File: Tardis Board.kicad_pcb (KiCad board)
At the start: 2 copper layers, 97.8 x 66 mm, 23 parts, among them J1 Conn_01x03_Female, Q1 IRLB8721PBF, SW1 SW_DIP_x01, SW2 SW_SPDT, SW3 SW_SPDT, SW4 SW_SPDT, SW5 SW_SPDT, SW6 SW_SPDT, SW7 SW_SPDT

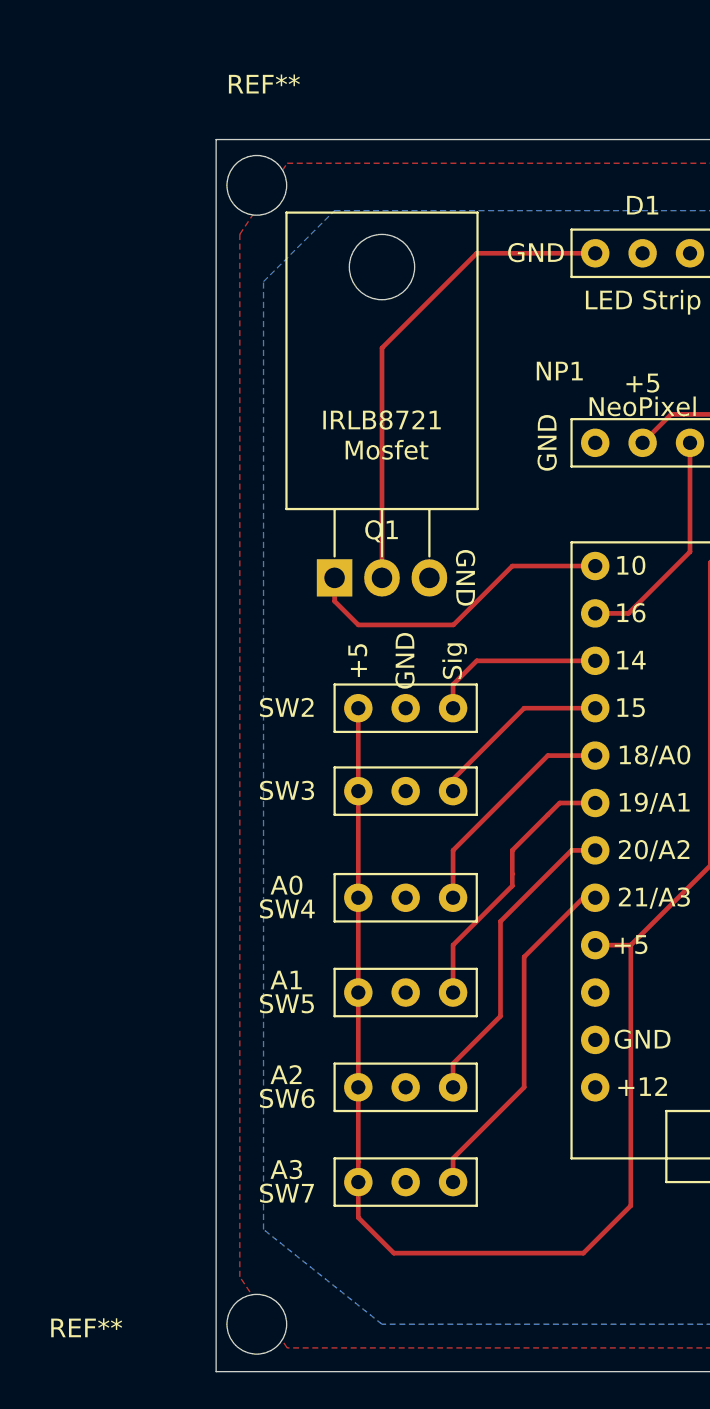
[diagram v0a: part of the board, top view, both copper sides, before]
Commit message: small updates
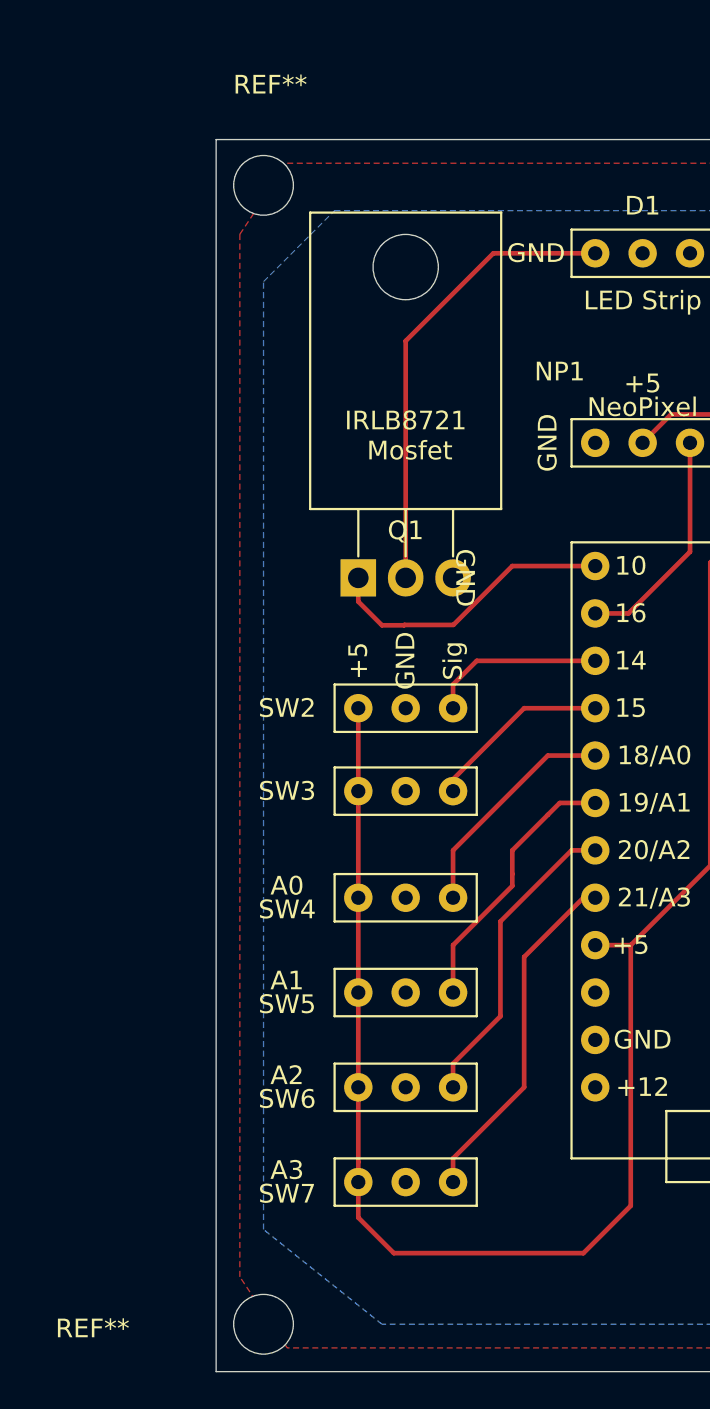
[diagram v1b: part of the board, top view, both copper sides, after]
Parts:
- moved Q1 1.27 mm to (92.7, 64.1)
- moved REF** 0.36 mm to (88.3, 103.7)
- moved REF** 0.36 mm to (88.0, 41.9)
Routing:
- net Net-(D1-Pad1): track 26.5 -> 24.8 mm
- net Net-(Ard1-Pad13): track 17.1 -> 15.8 mm
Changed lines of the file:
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@@
     (thickness 1.6)
     (drawings 100)
-    (tracks 81)
+    (tracks 82)
     (zones 0)
     (modules 23)
@@
     (add_net VCC)
   )
+  (module Package_TO_SOT_THT:TO-220-3_Horizontal_TabDown (layer F.Cu)
+    (at 92.71 64.135)
+    (descr "TO-220-3, Horizontal, RM 2.54mm, see https://www.vishay.com/docs/66542/to-220-1.pdf")
+    (tags "TO-220-3 Horizontal RM 2.54mm")
+    (fp_text reference Q1 (at 2.54 -2.54) (layer F.SilkS)
+      (effects (font (size 1 1) (thickness 0.15)))
+    )
+    (fp_text value IRLB8721PBF (at 2.54 2.5) (layer F.Fab)
+      (effects (font (size 1 1) (thickness 0.15)))
+    )
+    (fp_text user %R (at 2.54 -4.27) (layer F.Fab)
+      (effects (font (size 1 1) (thickness 0.15)))
+    )
+    (fp_line (start 7.79 -19.71) (end -2.71 -19.71) (layer F.CrtYd) (width 0.05))
+    (fp_line (start 7.79 1.25) (end 7.79 -19.71) (layer F.CrtYd) (width 0.05))
+    (fp_line (start -2.71 1.25) (end 7.79 1.25) (layer F.CrtYd) (width 0.05))
+    (fp_line (start -2.71 -19.71) (end -2.71 1.25) (layer F.CrtYd) (width 0.05))
+    (fp_line (start 5.08 -3.69) (end 5.08 -1.15) (layer F.SilkS) (width 0.12))
+    (fp_line (start 2.54 -3.69) (end 2.54 -1.15) (layer F.SilkS) (width 0.12))
+    (fp_line (start 0 -3.69) (end 0 -1.15) (layer F.SilkS) (width 0.12))
+    (fp_line (start 7.66 -19.58) (end 7.66 -3.69) (layer F.SilkS) (width 0.12))
+    (fp_line (start -2.58 -19.58) (end -2.58 -3.69) (layer F.SilkS) (width 0.12))
+    (fp_line (start -2.58 -19.58) (end 7.66 -19.58) (layer F.SilkS) (width 0.12))
+    (fp_line (start -2.58 -3.69) (end 7.66 -3.69) (layer F.SilkS) (width 0.12))
+    (fp_line (start 5.08 -3.81) (end 5.08 0) (layer F.Fab) (width 0.1))
+    (fp_line (start 2.54 -3.81) (end 2.54 0) (layer F.Fab) (width 0.1))
+    (fp_line (start 0 -3.81) (end 0 0) (layer F.Fab) (width 0.1))
+    (fp_line (start 7.54 -3.81) (end -2.46 -3.81) (layer F.Fab) (width 0.1))
+    (fp_line (start 7.54 -13.06) (end 7.54 -3.81) (layer F.Fab) (width 0.1))
+    (fp_line (start -2.46 -13.06) (end 7.54 -13.06) (layer F.Fab) (width 0.1))
+    (fp_line (start -2.46 -3.81) (end -2.46 -13.06) (layer F.Fab) (width 0.1))
+    (fp_line (start 7.54 -13.06) (end -2.46 -13.06) (layer F.Fab) (width 0.1))
+    (fp_line (start 7.54 -19.46) (end 7.54 -13.06) (layer F.Fab) (width 0.1))
+    (fp_line (start -2.46 -19.46) (end 7.54 -19.46) (layer F.Fab) (width 0.1))
+    (fp_line (start -2.46 -13.06) (end -2.46 -19.46) (layer F.Fab) (width 0.1))
+    (fp_circle (center 2.54 -16.66) (end 4.39 -16.66) (layer F.Fab) (width 0.1))
+    (pad 3 thru_hole oval (at 5.08 0) (size 1.905 2) (drill 1.1) (layers *.Cu *.Mask)
+      (net 2 GND))
+    (pad 2 thru_hole oval (at 2.54 0) (size 1.905 2) (drill 1.1) (layers *.Cu *.Mask)
+      (net 20 "Net-(D1-Pad1)"))
+    (pad 1 thru_hole rect (at 0 0) (size 1.905 2) (drill 1.1) (layers *.Cu *.Mask)
+      (net 7 "Net-(Ard1-Pad13)"))
+    (pad "" np_thru_hole oval (at 2.54 -16.66) (size 3.5 3.5) (drill 3.5) (layers *.Cu *.Mask))
+    (model ${KISYS3DMOD}/Package_TO_SOT_THT.3dshapes/TO-220-3_Horizontal_TabDown.wrl
+      (at (xyz 0 0 0))
+      (scale (xyz 1 1 1))
+      (rotate (xyz 0 0 0))
+    )
+  )
   (module Libraries:LED_CONNECTOR (layer F.Cu)
     (at 95.25 96.52)
@@
     (pad 1 thru_hole circle (at -3.81 35.56 180) (size 1.524 1.524) (drill 0.762) (layers *.Cu *.Mask)
       (net 4 VCC))
-  )
-  (module Package_TO_SOT_THT:TO-220-3_Horizontal_TabDown (layer F.Cu)
-    (at 91.44 64.135)
-    (descr "TO-220-3, Horizontal, RM 2.54mm, see https://www.vishay.com/docs/66542/to-220-1.pdf")
-    (tags "TO-220-3 Horizontal RM 2.54mm")
-    (fp_text reference Q1 (at 2.54 -2.54) (layer F.SilkS)
-      (effects (font (size 1 1) (thickness 0.15)))
-    )
-    (fp_text value IRLB8721PBF (at 2.54 2.5) (layer F.Fab)
-      (effects (font (size 1 1) (thickness 0.15)))
-    )
-    (fp_text user %R (at 2.54 -4.27) (layer F.Fab)
-      (effects (font (size 1 1) (thickness 0.15)))
-    )
-    (fp_line (start 7.79 -19.71) (end -2.71 -19.71) (layer F.CrtYd) (width 0.05))
-    (fp_line (start 7.79 1.25) (end 7.79 -19.71) (layer F.CrtYd) (width 0.05))
-    (fp_line (start -2.71 1.25) (end 7.79 1.25) (layer F.CrtYd) (width 0.05))
-    (fp_line (start -2.71 -19.71) (end -2.71 1.25) (layer F.CrtYd) (width 0.05))
-    (fp_line (start 5.08 -3.69) (end 5.08 -1.15) (layer F.SilkS) (width 0.12))
-    (fp_line (start 2.54 -3.69) (end 2.54 -1.15) (layer F.SilkS) (width 0.12))
-    (fp_line (start 0 -3.69) (end 0 -1.15) (layer F.SilkS) (width 0.12))
-    (fp_line (start 7.66 -19.58) (end 7.66 -3.69) (layer F.SilkS) (width 0.12))
-    (fp_line (start -2.58 -19.58) (end -2.58 -3.69) (layer F.SilkS) (width 0.12))
-    (fp_line (start -2.58 -19.58) (end 7.66 -19.58) (layer F.SilkS) (width 0.12))
-    (fp_line (start -2.58 -3.69) (end 7.66 -3.69) (layer F.SilkS) (width 0.12))
-    (fp_line (start 5.08 -3.81) (end 5.08 0) (layer F.Fab) (width 0.1))
-    (fp_line (start 2.54 -3.81) (end 2.54 0) (layer F.Fab) (width 0.1))
-    (fp_line (start 0 -3.81) (end 0 0) (layer F.Fab) (width 0.1))
-    (fp_line (start 7.54 -3.81) (end -2.46 -3.81) (layer F.Fab) (width 0.1))
-    (fp_line (start 7.54 -13.06) (end 7.54 -3.81) (layer F.Fab) (width 0.1))
-    (fp_line (start -2.46 -13.06) (end 7.54 -13.06) (layer F.Fab) (width 0.1))
-    (fp_line (start -2.46 -3.81) (end -2.46 -13.06) (layer F.Fab) (width 0.1))
-    (fp_line (start 7.54 -13.06) (end -2.46 -13.06) (layer F.Fab) (width 0.1))
-    (fp_line (start 7.54 -19.46) (end 7.54 -13.06) (layer F.Fab) (width 0.1))
-    (fp_line (start -2.46 -19.46) (end 7.54 -19.46) (layer F.Fab) (width 0.1))
-    (fp_line (start -2.46 -13.06) (end -2.46 -19.46) (layer F.Fab) (width 0.1))
-    (fp_circle (center 2.54 -16.66) (end 4.39 -16.66) (layer F.Fab) (width 0.1))
-    (pad 3 thru_hole oval (at 5.08 0) (size 1.905 2) (drill 1.1) (layers *.Cu *.Mask)
-      (net 2 GND))
-    (pad 2 thru_hole oval (at 2.54 0) (size 1.905 2) (drill 1.1) (layers *.Cu *.Mask)
-      (net 20 "Net-(D1-Pad1)"))
-    (pad 1 thru_hole rect (at 0 0) (size 1.905 2) (drill 1.1) (layers *.Cu *.Mask)
-      (net 7 "Net-(Ard1-Pad13)"))
-    (pad "" np_thru_hole oval (at 2.54 -16.66) (size 3.5 3.5) (drill 3.5) (layers *.Cu *.Mask))
-    (model ${KISYS3DMOD}/Package_TO_SOT_THT.3dshapes/TO-220-3_Horizontal_TabDown.wrl
-      (at (xyz 0 0 0))
-      (scale (xyz 1 1 1))
-      (rotate (xyz 0 0 0))
-    )
   )
   (module Symbol:OSHW-Logo2_7.3x6mm_SilkScreen (layer F.Cu)
@@
     (pad 22 thru_hole circle (at 10.16 0) (size 1.524 1.524) (drill 0.762) (layers *.Cu *.Mask)
       (net 39 /5v))
+    (model "${KIPRJMOD}/Sound Board Final.stp"
+      (offset (xyz 1 -14.5 14))
+      (scale (xyz 1 1 1))
+      (rotate (xyz 0 0 -90))
+    )
   )
   (module Libraries:ArduinoProMicro (layer F.Cu)
@@
     (pad 1 thru_hole circle (at -7.62 0 180) (size 1.524 1.524) (drill 0.762) (layers *.Cu *.Mask)
       (net 19 "Net-(Ard1-Pad1)"))
+    (model "${KIPRJMOD}/Not the Sound.stp"
+      (offset (xyz 1 -16 12))
+      (scale (xyz 1 1 1))
+      (rotate (xyz 0 0 -90))
+    )
   )
   (module MountingHole:MountingHole_3.2mm_M3 (layer F.Cu)
@@
   )
   (module MountingHole:MountingHole_3.2mm_M3 (layer F.Cu)
-    (at 87.99 103.74)
+    (at 88.35 103.74)
     (descr "Mounting Hole 3.2mm, no annular, M3")
     (tags "mounting hole 3.2mm no annular m3")
@@
   )
   (module MountingHole:MountingHole_3.2mm_M3 (layer F.Cu)
-    (at 87.63 41.91)
+    (at 87.99 41.91)
     (descr "Mounting Hole 3.2mm, no annular, M3")
     (tags "mounting hole 3.2mm no annular m3")
@@
     (effects (font (size 1 1) (thickness 0.15)))
   )
-  (gr_text "IRLB8721\n Mosfet" (at 93.98 56.515) (layer F.SilkS)
+  (gr_text "IRLB8721\n Mosfet" (at 95.25 56.515) (layer F.SilkS)
     (effects (font (size 1 1) (thickness 0.15)))
   )
@@
   (segment (start 105.41 66.04) (end 107.188 66.04) (width 0.25) (layer F.Cu) (net 6))
   (segment (start 107.188 66.04) (end 110.49 62.738) (width 0.25) (layer F.Cu) (net 6))
-  (segment (start 91.44 64.8175) (end 91.44 64.77) (width 0.25) (layer F.Cu) (net 7))
-  (segment (start 91.44 65.385) (end 92.71 66.655) (width 0.25) (layer F.Cu) (net 7))
-  (segment (start 91.44 64.135) (end 91.44 65.385) (width 0.25) (layer F.Cu) (net 7))
-  (segment (start 92.71 66.655) (end 97.81 66.655) (width 0.25) (layer F.Cu) (net 7))
   (segment (start 100.965 63.5) (end 105.41 63.5) (width 0.25) (layer F.Cu) (net 7))
   (segment (start 97.81 66.655) (end 100.965 63.5) (width 0.25) (layer F.Cu) (net 7))
+  (segment (start 95.1825 66.655) (end 95.1625 66.675) (width 0.25) (layer F.Cu) (net 7))
+  (segment (start 97.81 66.655) (end 95.1825 66.655) (width 0.25) (layer F.Cu) (net 7))
+  (segment (start 95.1625 66.675) (end 93.98 66.675) (width 0.25) (layer F.Cu) (net 7))
+  (segment (start 92.71 65.405) (end 92.71 64.135) (width 0.25) (layer F.Cu) (net 7))
+  (segment (start 93.98 66.675) (end 92.71 65.405) (width 0.25) (layer F.Cu) (net 7))
   (segment (start 120.65 63.5) (end 125.73 63.5) (width 0.25) (layer F.Cu) (net 8))
   (segment (start 120.65 66.04) (end 125.73 66.04) (width 0.25) (layer F.Cu) (net 9))
@@
   (segment (start 120.65 78.74) (end 125.73 78.74) (width 0.25) (layer F.Cu) (net 14))
   (segment (start 120.65 81.28) (end 125.73 81.28) (width 0.25) (layer F.Cu) (net 15))
-  (segment (start 99.06 46.736) (end 105.41 46.736) (width 0.25) (layer F.Cu) (net 20))
-  (segment (start 93.98 64.77) (end 93.98 51.816) (width 0.25) (layer F.Cu) (net 20))
-  (segment (start 93.98 51.816) (end 99.06 46.736) (width 0.25) (layer F.Cu) (net 20))
+  (segment (start 99.949 46.736) (end 105.41 46.736) (width 0.25) (layer F.Cu) (net 20))
+  (segment (start 95.25 64.135) (end 95.25 51.435) (width 0.25) (layer F.Cu) (net 20))
+  (segment (start 95.25 51.435) (end 99.949 46.736) (width 0.25) (layer F.Cu) (net 20))
   (segment (start 97.79 96.52) (end 97.79 95.25) (width 0.25) (layer F.Cu) (net 29))
   (segment (start 97.79 95.25) (end 101.6 91.44) (width 0.25) (layer F.Cu) (net 29))
